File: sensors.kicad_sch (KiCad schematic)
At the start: 22 parts, among them Q1 TEFT4300, Q2 TEFT4300, Q5 Q_NMOS_DGS

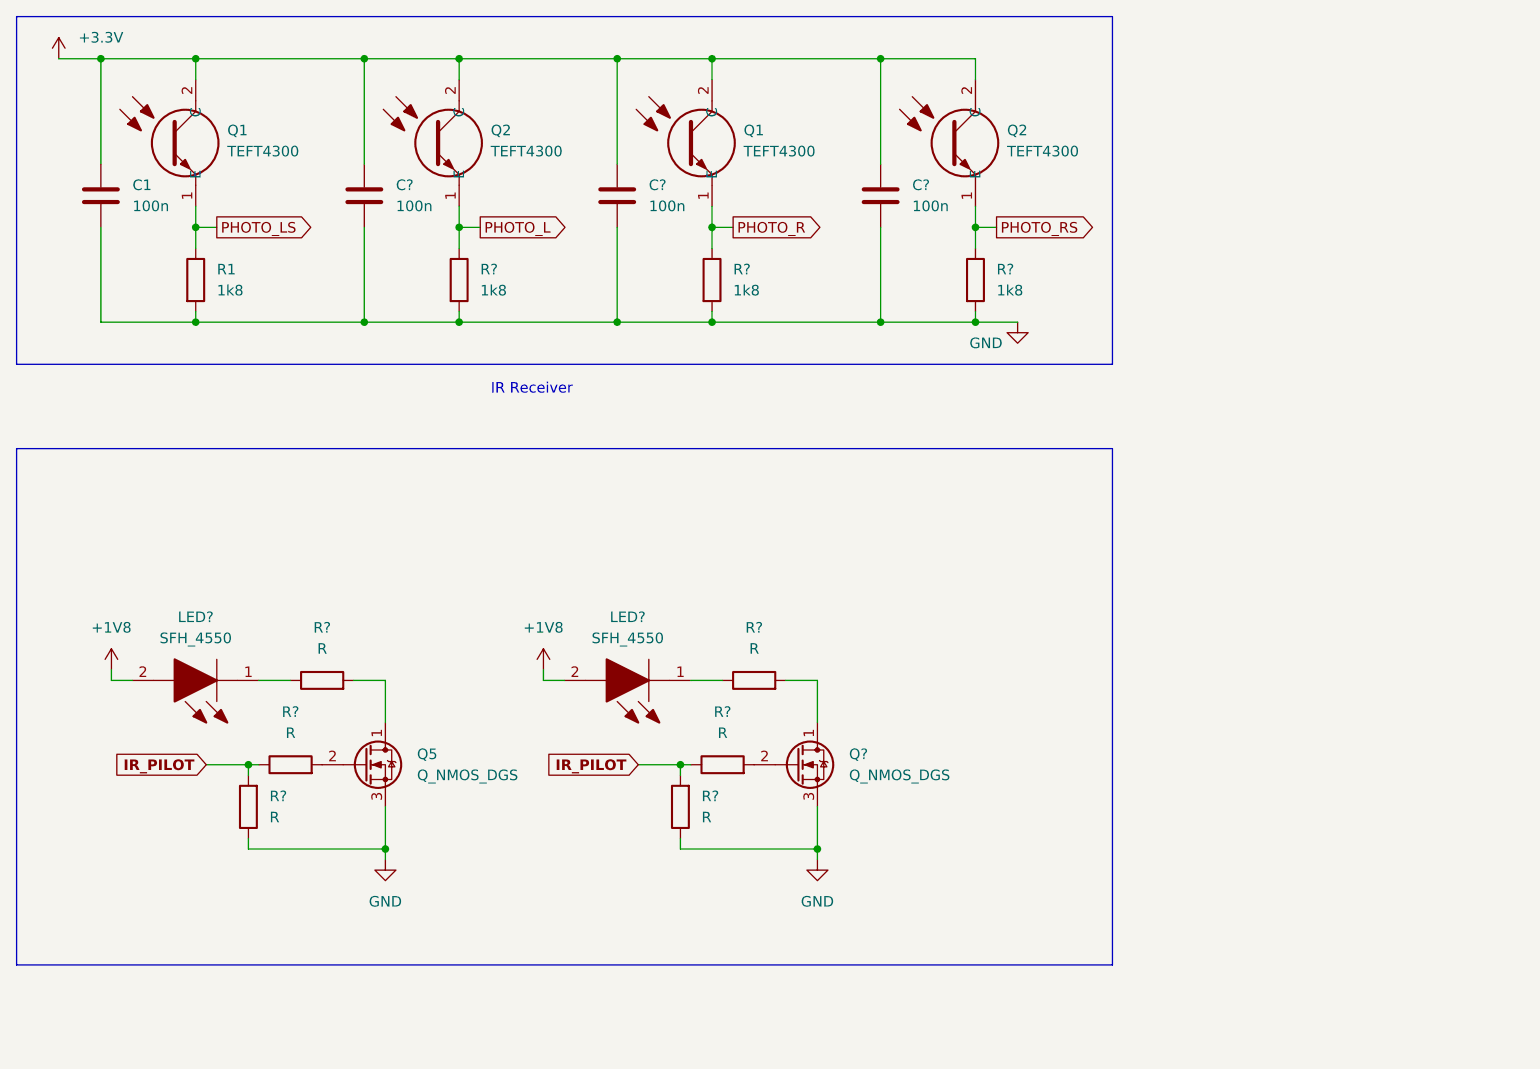
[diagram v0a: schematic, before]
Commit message: finish IR transmitters
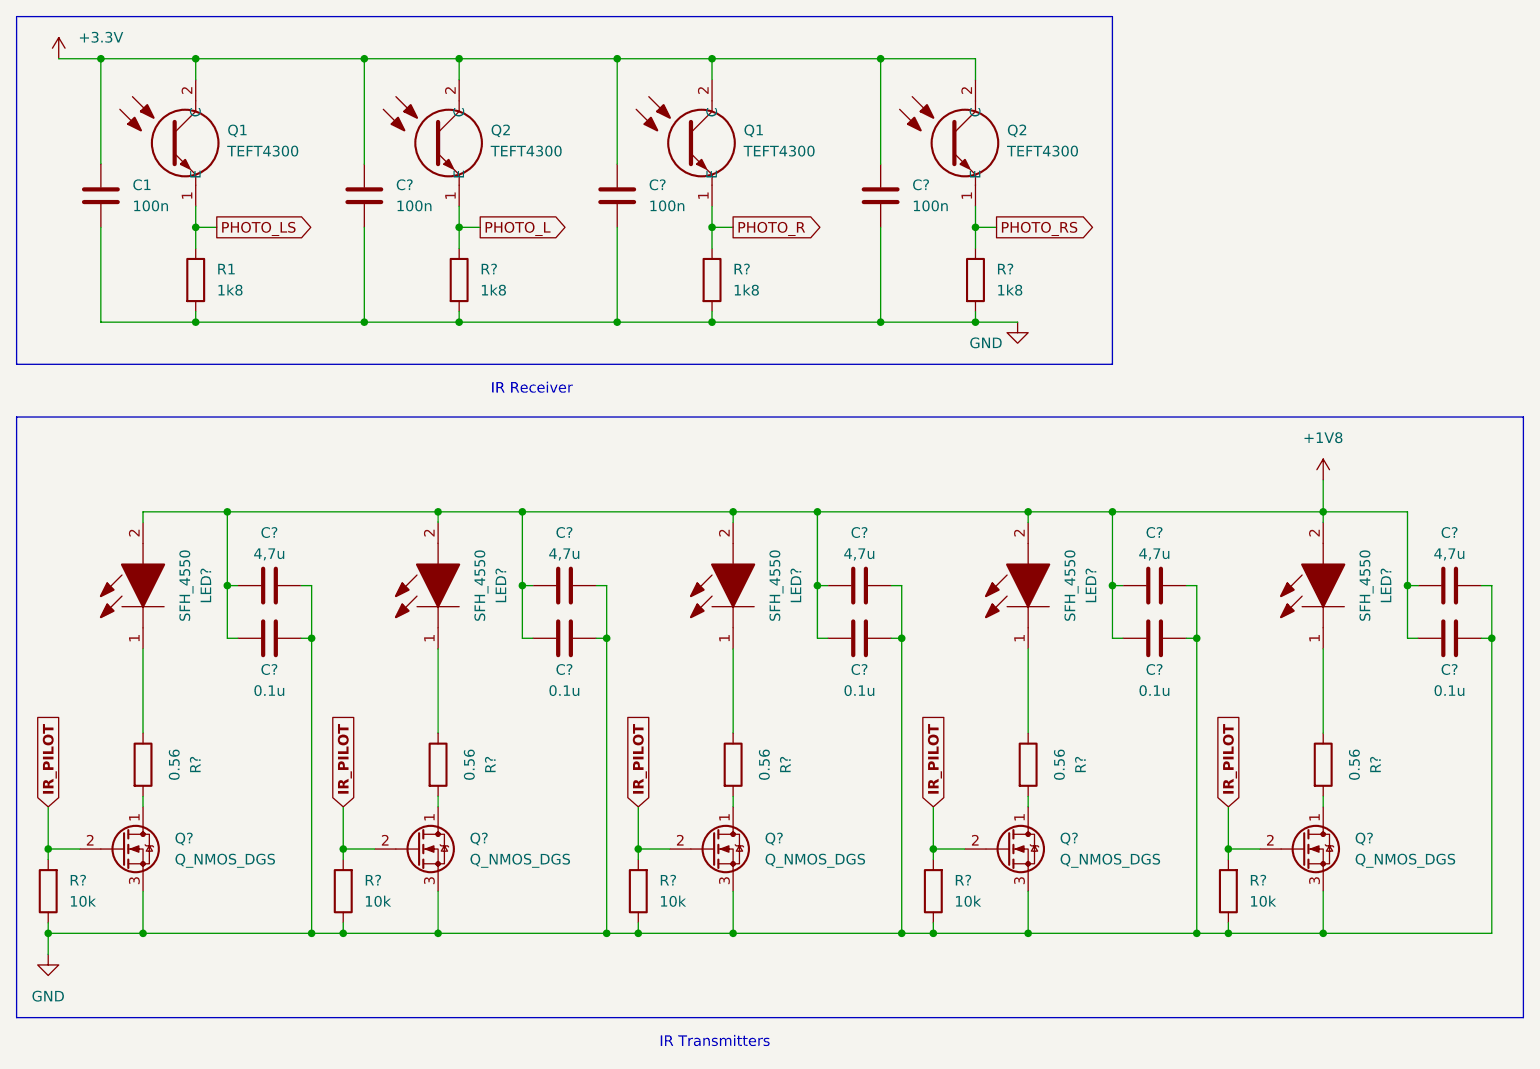
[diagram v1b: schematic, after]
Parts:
- removed LED?: SFH_4550, SFH4550, symbol SFH_4550:SFH_4550
- removed Q5: Q_NMOS_DGS, symbol Device:Q_NMOS_DGS
- removed R? (x4): R, symbol Device:R
- added C? (x5): 0.1u, symbol Device:C
- added C? (x5): 4,7u, symbol Device:C
- added LED? (x4): SFH_4550, SFH4550, symbol SFH_4550:SFH_4550
- added Q? (x4): Q_NMOS_DGS, symbol Device:Q_NMOS_DGS
- added R? (x4): 10k, symbol Device:R
- added R? (x4): 0.56, symbol Device:R
- R?: value R -> 10k
- R?: value R -> 0.56
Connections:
- net +1V8: now also C?.1, C?.1, C?.1, C?.1, C?.1, C?.1, C?.1, C?.1, C?.1, C?.1, LED?.2, LED?.2, LED?.2, LED?.2
- net GND: now also C?.2, C?.2, C?.2, C?.2, C?.2, C?.2, C?.2, C?.2, C?.2, C?.2, Q?.3 (S), Q?.3 (S), Q?.3 (S), Q?.3 (S), R?.1, R?.1, R?.1, R?.1
- net IR_PILOT: now also Q?.2 (G), Q?.2 (G), Q?.2 (G), Q?.2 (G), Q?.2 (G), R?.2, R?.2, R?.2, R?.2
- new net: LED?.1, R?.1 (x4)
- new net: Q?.1 (D), R?.2 (x4)
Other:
- note added: "IR Transmitters"
- moved on the sheet: LED?, Q?, R?
